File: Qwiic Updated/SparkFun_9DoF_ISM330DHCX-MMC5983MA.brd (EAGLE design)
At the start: 25.4 x 25.4 mm, 59 parts, among them J1 QWIIC_RIGHT_ANGLE, J2 QWIIC_RIGHT_ANGLE, U1 ISM330DHCX, U2 MMC5983MA_QFN16

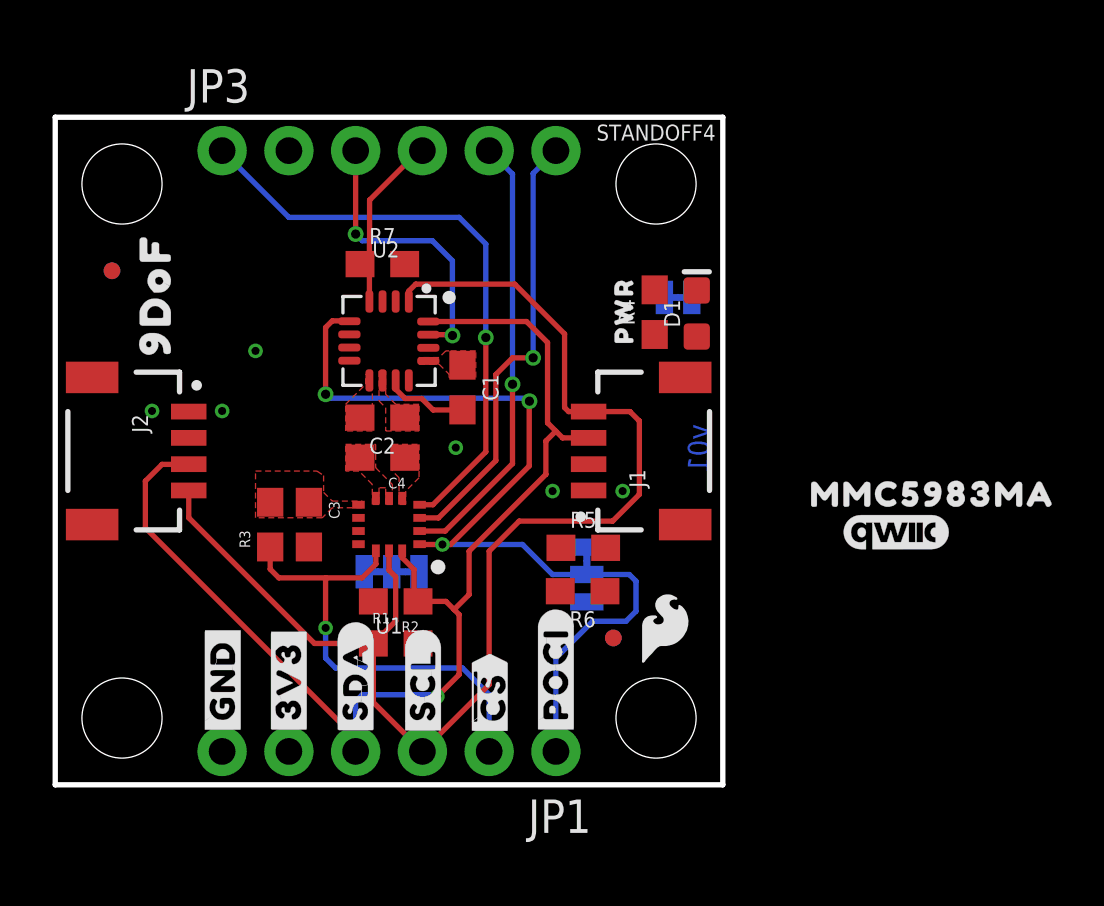
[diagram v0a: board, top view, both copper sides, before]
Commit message: More updates to the routing
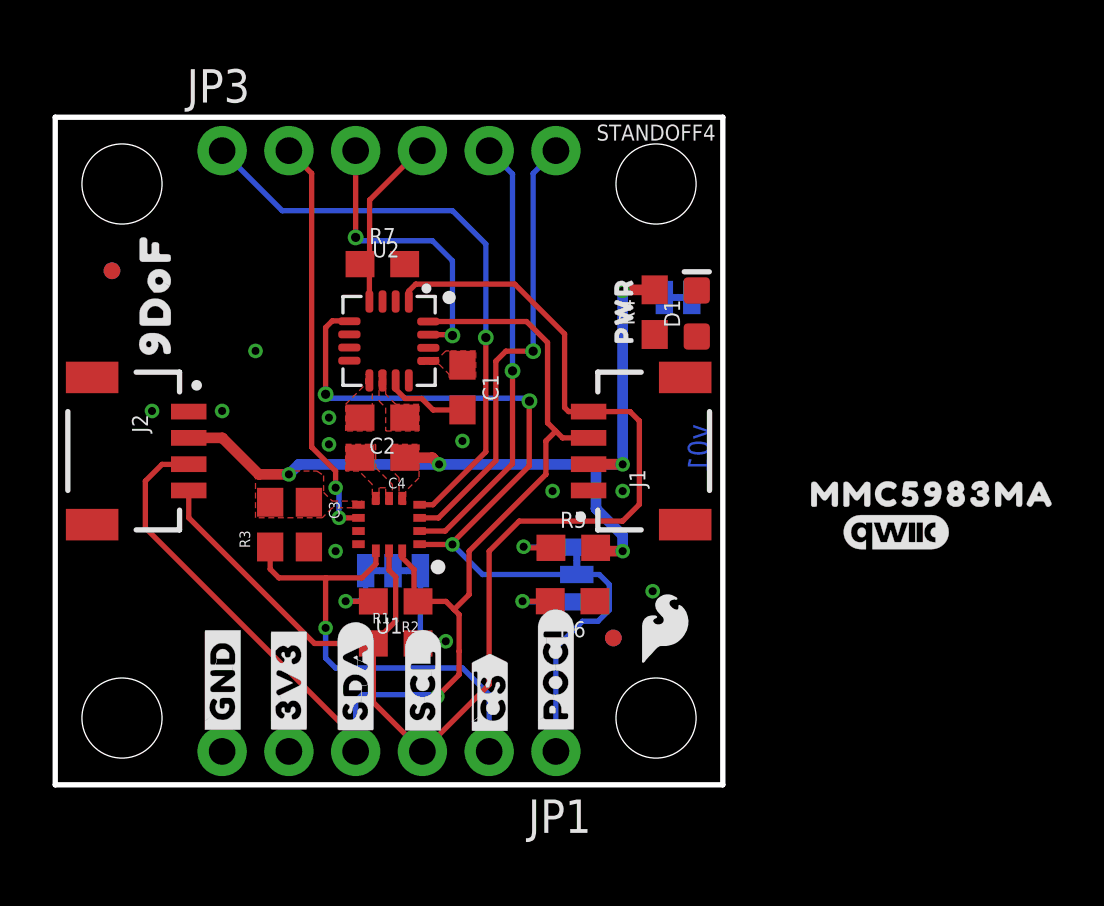
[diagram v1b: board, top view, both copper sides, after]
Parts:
- moved R6 0.54 mm to (19.7, 6.99)
- moved 6DOF_ADDR 0.38 mm to (19.8, 8.00)
- moved R5 0.38 mm to (19.7, 9.02)
- moved I2C_PU 0.06 mm to (12.9, 8.15), turned to 0 degrees
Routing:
- net 3.3V: track 0.00 -> 32.8 mm, vias 0 -> 5
- net ISM_INT2: track 0.00 -> 15.5 mm, vias 0 -> 2
- net N$5: track 0.00 -> 4.62 mm, vias 0 -> 1
- net N$7: track 0.00 -> 3.13 mm, vias 0 -> 1
- net N$1: track 0.00 -> 3.08 mm, vias 0 -> 1
- net N$6: track 0.00 -> 2.83 mm, vias 0 -> 1
- net POCI/SA0: track 35.7 -> 33.5 mm
- net GND: vias 6 -> 10
